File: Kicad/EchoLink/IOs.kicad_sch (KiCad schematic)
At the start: 8 parts, among them J2 Conn_01x09, J4 Conn_01x06_Pin, J5 Conn_01x03, J6 Conn_01x07_Pin, J7 Conn_01x07_Pin, J8 Conn_01x05_Pin

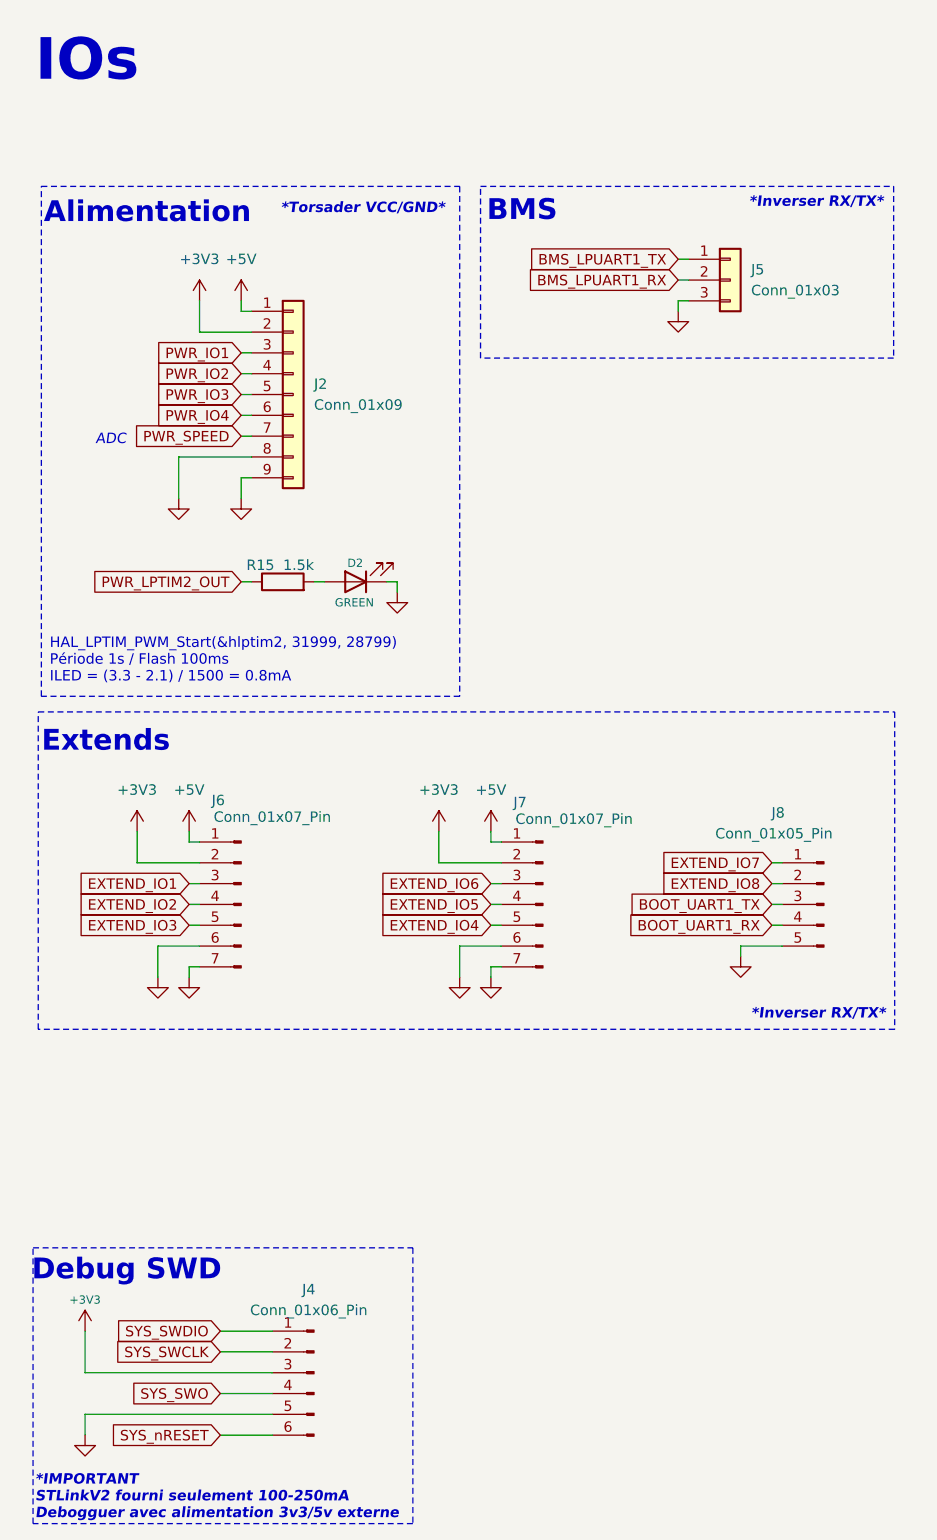
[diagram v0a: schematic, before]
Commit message: wip: add missing footprints
- connectors missing
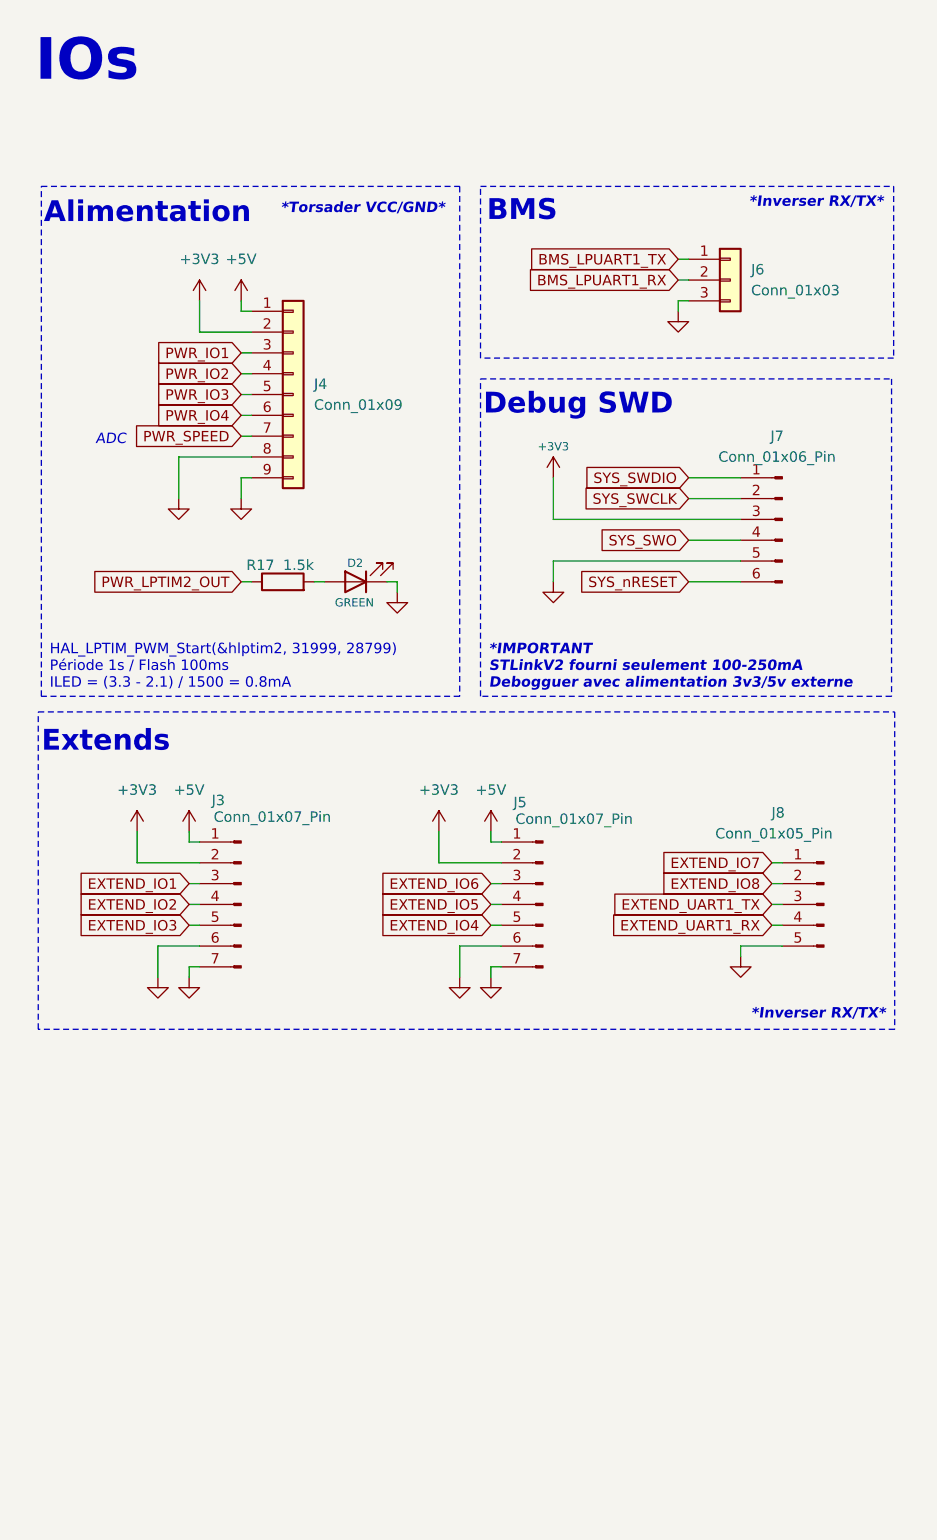
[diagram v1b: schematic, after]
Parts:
- D2: footprint (none) -> Resistor_SMD:R_0603_1608Metric
- J3: renamed from J6; footprint (none) -> Connector_PinHeader_2.54mm:PinHeader_1x07_P2.54mm_Vertical
- J5: renamed from J7; footprint (none) -> Connector_PinHeader_2.54mm:PinHeader_1x07_P2.54mm_Vertical
- J6: renamed from J5; footprint Connector_RJ:RJ45_Abracon_ARJP11A-MA_Horizontal -> (none)
- J8: footprint (none) -> Connector_PinHeader_2.54mm:PinHeader_1x05_P2.54mm_Vertical
- renumbered J2 to J4, J4 to J7, R15 to R17
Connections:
- net BOOT_UART1_RX renamed EXTEND_UART1_RX
- net BOOT_UART1_TX renamed EXTEND_UART1_TX
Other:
- moved on the sheet: J7
